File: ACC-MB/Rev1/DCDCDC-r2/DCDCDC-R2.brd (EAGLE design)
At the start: 89.8 x 62 mm, 21 parts, among them X2 5566-4

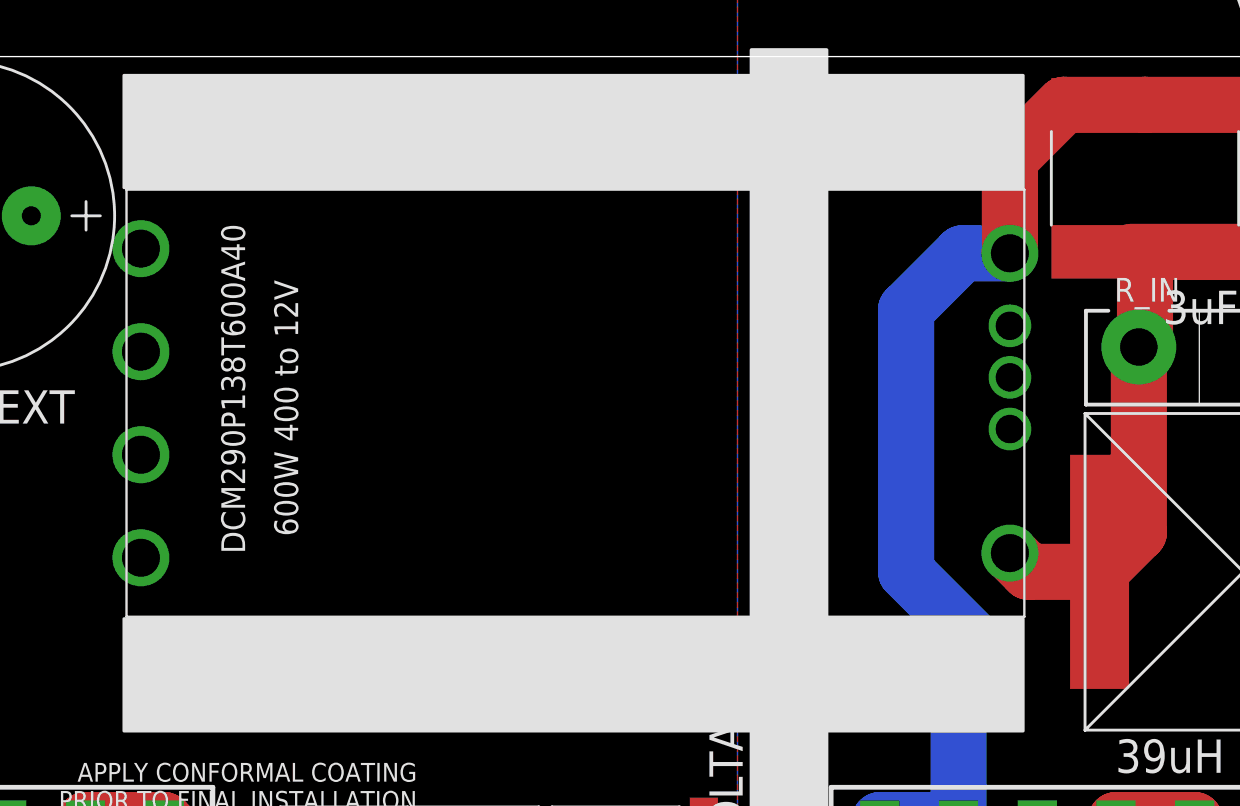
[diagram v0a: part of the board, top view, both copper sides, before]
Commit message: update
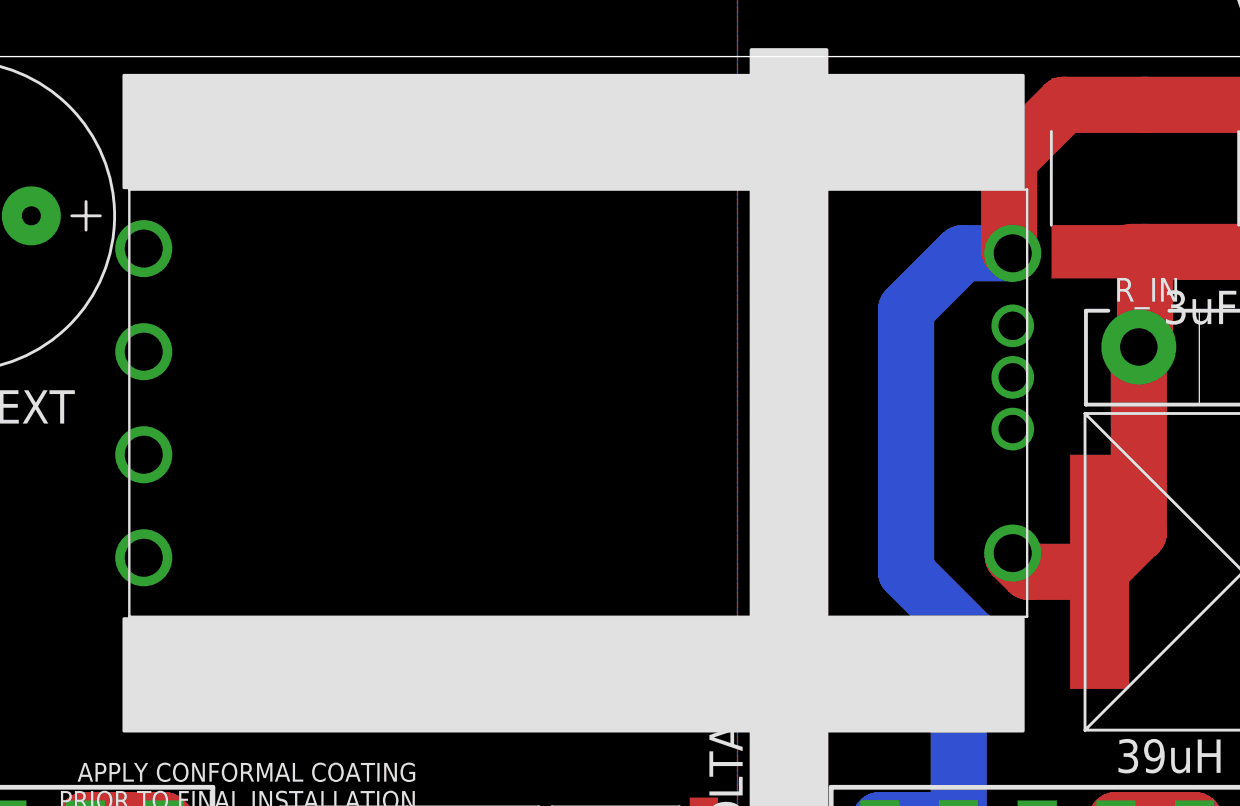
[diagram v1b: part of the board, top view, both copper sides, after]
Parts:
- removed DCM290P138T600A40: 600W 400 to 12V, ACC-MB-R0:VICOR_CHIP_HEATSINK
- added U$8: VICOR_CHIP_WITH_HEATSINK, ACC-MB-R0:VICOR_CHIP_HEATSINK
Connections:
- net DCDC_OUT: now also U$8.OUT+_1, U$8.OUT+_2; no longer DCM290P138T600A40.OUT+_1, DCM290P138T600A40.OUT+_2
- net GND: now also U$8.OUT-_1, U$8.OUT-_2; no longer DCM290P138T600A40.OUT-_1, DCM290P138T600A40.OUT-_2
- net N$3: now also U$8.IN+; no longer DCM290P138T600A40.IN+
- net V-: now also U$8.IN-; no longer DCM290P138T600A40.IN-
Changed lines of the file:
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@@
 </layers>
 <board>
-<fusionsync huburn="a.YnVzaW5lc3M6bXl1d28yNA" projecturn="a.YnVzaW5lc3M6bXl1d28yNCNEMjAxOTA5MTgyMTU4NTEzMzE" f3durn="urn:adsk.wipprod:dm.lineage:U_-0G6fwRzqBO_3Lu0JAiA" pcbguid="ece931dd-8bcb-4325-baf8-111b939a3e73" lastpulledtime="" lastsyncedchangeguid="07639025-2a20-f54b-1a95-872b400ec342"/>
+<fusionsync huburn="a.YnVzaW5lc3M6bXl1d28yNA" projecturn="a.YnVzaW5lc3M6bXl1d28yNCNEMjAxOTA5MTgyMTU4NTEzMzE" f3durn="urn:adsk.wipprod:dm.lineage:U_-0G6fwRzqBO_3Lu0JAiA" pcbguid="ece931dd-8bcb-4325-baf8-111b939a3e73" lastpulledtime="" lastsyncedchangeguid="cb0f9be5-9551-2798-ee30-78990f0e4cb6"/>
 <plain>
 <wire x1="92.5" y1="66.5" x2="2.75" y2="66.5" width="0" layer="20"/>
@@
 </autorouter>
 <elements>
-<element name="DCM290P138T600A40" library="ACC-MB-R0" library_urn="urn:adsk.eagle:library:13324935" package="VICOR_CHIP_HEATSINK" package3d_urn="urn:adsk.eagle:package:13209498/1" value="600W 400 to 12V" x="44.35" y="48" smashed="yes" rot="R180">
-<attribute name="NAME" x="25.45" y="57.57" size="1.27" layer="21" rot="R270"/>
-<attribute name="VALUE" x="28.28" y="54.57" size="1.27" layer="21" rot="R270"/>
-</element>
 <element name="U$4" library="ACC-MB-R0" library_urn="urn:adsk.eagle:library:13324935" package="SOT23" package3d_urn="urn:adsk.eagle:package:13209499/1" value="RK7002BMT116" x="44.4" y="11.45" smashed="yes">
 <attribute name="NAME" x="42.495" y="13.355" size="1.27" layer="25"/>
@@
 <attribute name="SPICEPREFIX" value="R" x="7" y="42.5" size="1.778" layer="28" rot="MR270" display="off"/>
 </element>
+<element name="U$8" library="ACC-MB-R0" library_urn="urn:adsk.eagle:library:13208985" package="VICOR_CHIP_HEATSINK" package3d_urn="urn:adsk.eagle:package:13209498/2" value="VICOR_CHIP_WITH_HEATSINK" x="44.5" y="48" rot="R180"/>
 </elements>
 <signals>
@@
 <contactref element="R2" pad="1"/>
 <contactref element="U$5" pad="2"/>
-<contactref element="DCM290P138T600A40" pad="OUT-_1"/>
-<contactref element="DCM290P138T600A40" pad="OUT-_2"/>
 <polygon width="1" layer="16">
 <vertex x="53" y="-10.5"/>
@@
 <contactref element="U$2" pad="5"/>
 <contactref element="R4" pad="1"/>
+<contactref element="U$8" pad="OUT-_1"/>
+<contactref element="U$8" pad="OUT-_2"/>
+<wire x1="7" y1="43.45" x2="7.69" y2="58" width="0" layer="19" extent="16-16"/>
+<wire x1="5.6" y1="20.25" x2="7" y2="43.45" width="0" layer="19" extent="16-16"/>
+<wire x1="9.8" y1="20.25" x2="5.6" y2="20.25" width="0" layer="19" extent="1-1"/>
+<wire x1="14" y1="20.25" x2="9.8" y2="20.25" width="0" layer="19" extent="1-1"/>
+<wire x1="18.2" y1="20.25" x2="14" y2="20.25" width="0" layer="19" extent="1-1"/>
+<wire x1="22.4" y1="20.25" x2="18.2" y2="20.25" width="0" layer="19" extent="1-1"/>
+<wire x1="28.4" y1="6.75" x2="22.4" y2="20.25" width="0" layer="19" extent="1-1"/>
+<wire x1="32.6" y1="6.75" x2="28.4" y2="6.75" width="0" layer="19" extent="1-1"/>
+<wire x1="41.2" y1="10.4" x2="32.6" y2="6.75" width="0" layer="19" extent="1-1"/>
+<wire x1="21.31" y1="45.25" x2="28.4" y2="6.75" width="0" layer="19" extent="1-1"/>
+<wire x1="21.31" y1="56.25" x2="21.31" y2="45.25" width="0" layer="19" extent="1-1"/>
 </signal>
 <signal name="V+" class="1">
@@
 <contactref element="CFILTER_1" pad="P$2"/>
 <contactref element="CFILTER_2" pad="P$2"/>
-<contactref element="DCM290P138T600A40" pad="IN-"/>
 <wire x1="73.075" y1="63.925" x2="74.75" y2="63.925" width="1" layer="1"/>
-<wire x1="67.54" y1="56" x2="67.54" y2="60.96" width="3" layer="1"/>
 <wire x1="67.54" y1="60.96" x2="67.5" y2="61" width="3" layer="1"/>
 <wire x1="67.5" y1="61" x2="70.425" y2="63.925" width="3" layer="1"/>
 <wire x1="70.425" y1="63.925" x2="74.75" y2="63.925" width="3" layer="1"/>
 <wire x1="74.75" y1="63.925" x2="86" y2="63.925" width="3" layer="1"/>
-<wire x1="65" y1="56" x2="67.54" y2="56" width="3" layer="16"/>
 <wire x1="65.5" y1="35.5" x2="62" y2="39" width="3" layer="16"/>
 <wire x1="62" y1="39" x2="62" y2="53" width="3" layer="16"/>
-<wire x1="62" y1="53" x2="65" y2="56" width="3" layer="16"/>
+<wire x1="65" y1="56" x2="62" y2="53" width="3" layer="16"/>
 <contactref element="U$1" pad="4"/>
 <contactref element="U$1" pad="5"/>
@@
 <wire x1="64.8" y1="32.25980625" x2="65.5" y2="32.95980625" width="3" layer="16"/>
 <wire x1="65.5" y1="32.95980625" x2="65.5" y2="35.5" width="3" layer="16"/>
+<contactref element="U$8" pad="IN-"/>
+<wire x1="67.69" y1="56" x2="67.5" y2="56.19" width="3" layer="1"/>
+<wire x1="67.5" y1="56.19" x2="67.5" y2="61" width="3" layer="1"/>
+<wire x1="67.69" y1="56" x2="65" y2="56" width="3" layer="16"/>
 </signal>
 <signal name="+12V" class="1">
@@
 <signal name="N$3" class="1">
 <contactref element="L_IN" pad="P$2"/>
-<contactref element="DCM290P138T600A40" pad="IN+"/>
 <contactref element="CFILTER_1" pad="P$1"/>
 <contactref element="CFILTER_2" pad="P$1"/>
@@
 <wire x1="74.42" y1="51" x2="74.42" y2="41.095" width="3" layer="1"/>
 <wire x1="74.42" y1="41.095" x2="72.325" y2="39" width="3" layer="1"/>
-<wire x1="72.325" y1="39" x2="68.54" y2="39" width="3" layer="1"/>
-<wire x1="68.54" y1="39" x2="67.54" y2="40" width="3" layer="1"/>
+<wire x1="68.54" y1="39" x2="72.325" y2="39" width="3" layer="1"/>
+<contactref element="U$8" pad="IN+"/>
+<wire x1="67.69" y1="40" x2="67.69" y2="39.85" width="3" layer="1"/>
+<wire x1="67.69" y1="39.85" x2="68.54" y2="39" width="3" layer="1"/>
 </signal>
 <signal name="V+_FUSED" class="1">
@@
 </signal>
 <signal name="DCDC_OUT" class="1">
-<contactref element="DCM290P138T600A40" pad="OUT+_1"/>
-<contactref element="DCM290P138T600A40" pad="OUT+_2"/>
 <contactref element="COUT_EXT" pad="+"/>
 <polygon width="1" layer="1">
@@
 <contactref element="U$3" pad="1"/>
 <contactref element="U$3" pad="3"/>
+<contactref element="U$8" pad="OUT+_1"/>
+<contactref element="U$8" pad="OUT+_2"/>
+<wire x1="48.405" y1="25.215" x2="51.2" y2="26.3" width="0" layer="19" extent="1-1"/>
+<wire x1="47.135" y1="25.215" x2="48.405" y2="25.215" width="0" layer="19" extent="1-1"/>
+<wire x1="45.865" y1="25.215" x2="47.135" y2="25.215" width="0" layer="19" extent="1-1"/>
+<wire x1="40.905" y1="25.215" x2="45.865" y2="25.215" width="0" layer="19" extent="1-1"/>
+<wire x1="39.635" y1="25.215" x2="40.905" y2="25.215" width="0" layer="19" extent="1-1"/>
+<wire x1="38.365" y1="25.215" x2="39.635" y2="25.215" width="0" layer="19" extent="1-1"/>
+<wire x1="33.905" y1="25.215" x2="38.365" y2="25.215" width="0" layer="19" extent="1-1"/>
+<wire x1="32.635" y1="25.215" x2="33.905" y2="25.215" width="0" layer="19" extent="1-1"/>
+<wire x1="31.365" y1="25.215" x2="32.635" y2="25.215" width="0" layer="19" extent="1-1"/>
+<wire x1="15.31" y1="58" x2="31.365" y2="25.215" width="0" layer="19" extent="1-1"/>
+<wire x1="21.31" y1="39.75" x2="31.365" y2="25.215" width="0" layer="19" extent="1-1"/>
+<wire x1="21.31" y1="50.75" x2="21.31" y2="39.75" width="0" layer="19" extent="1-1"/>
 </signal>
 <signal name="N$4" class="1">
